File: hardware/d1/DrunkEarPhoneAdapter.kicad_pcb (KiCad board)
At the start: 4 copper layers, 50 x 35 mm, 185 parts, among them J3 SWD, J4 UART, Q1 CSD17577Q3A, Q2 CSD17577Q3A, Q3 DMG1012T-7, SW1 SSSS811101, SW2 DSHP04TS-S, U1 CS43131-CNZR, U10 BLM15PX601SN1D, U11 TPS7A2033PDBVR, U12 TPS7A2018PDBVR, U13 TPS7A2018PDBVR, U14 BLM15PX601SN1D, U15 ESDA25P35-1U1M, U16 ESDA25P35-1U1M, U17 SN74LVC1G32DBVR, U18 TPS22917DBVR, U19 TPS22917DBVR, U2 STM32G0B1VCT6, U20 SN74AVC4T774RSVR, U21 TCA9406DCUR, U3 TS3USB221RSER, U4 TCPP03-M20, U5 TCPP03-M20, U6 ES8327, U7 TPS7A2018PDBVR, U8 TPS7A2033PDBVR, U9 TPS560430XFDBVR, X1 22.5792MHz, X3 24.576MHz

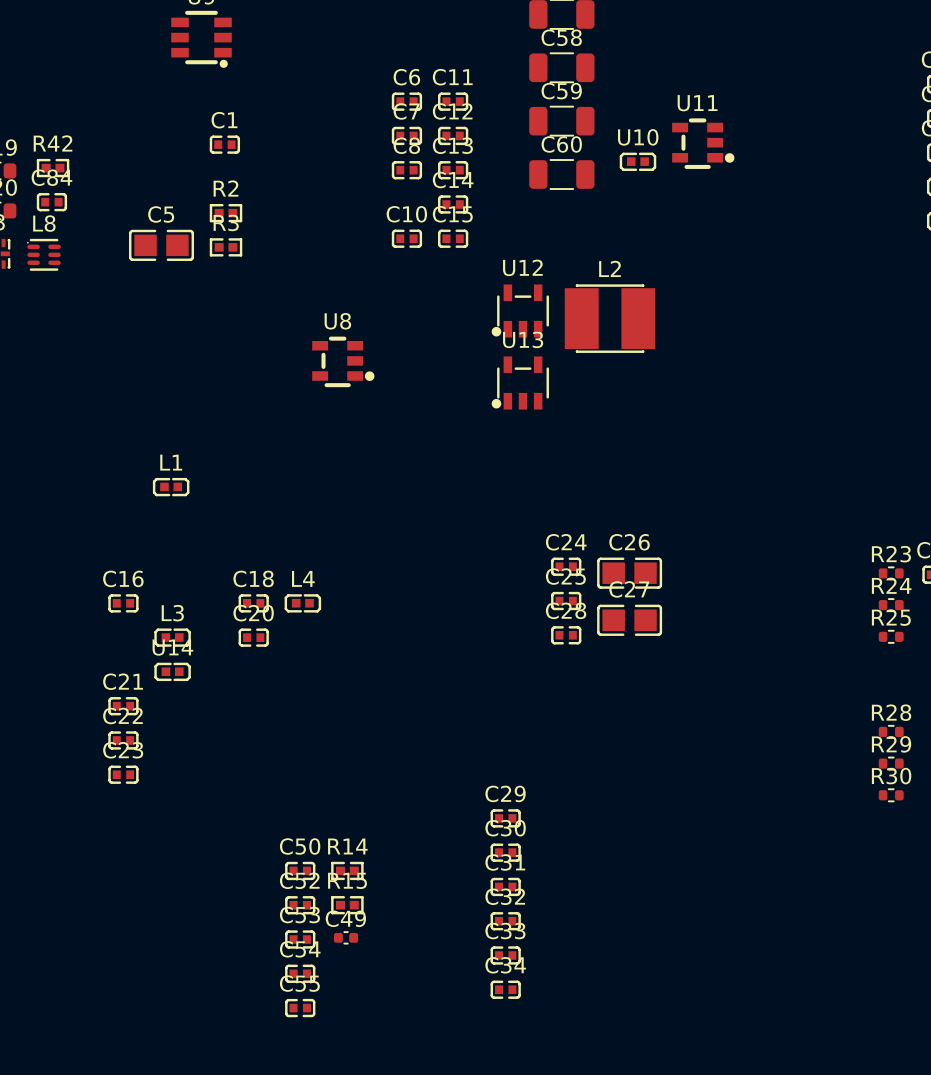
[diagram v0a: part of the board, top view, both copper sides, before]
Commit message: Fix Caps
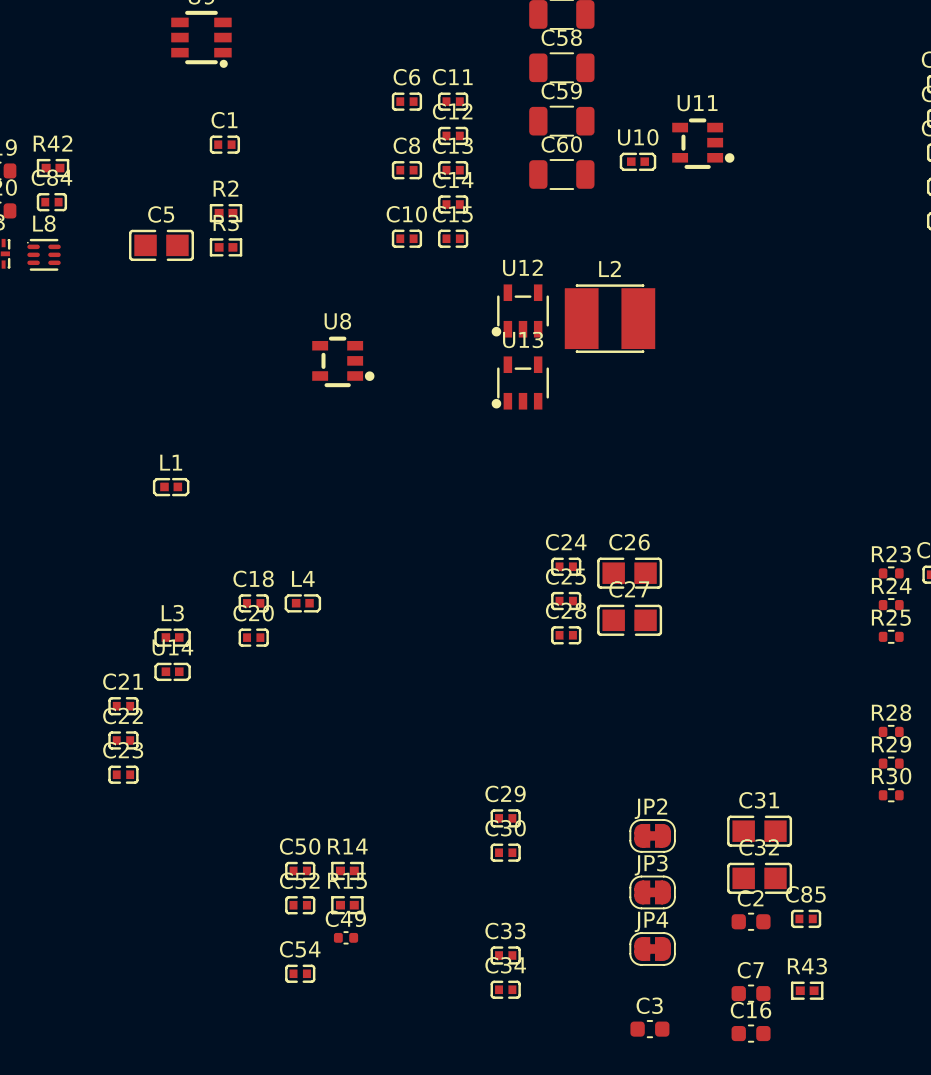
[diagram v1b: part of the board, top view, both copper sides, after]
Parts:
- removed C53, C55: 4.7uF 10V X5R, JLCImport:CL05A475MP5NRNC
- added C2: 4.7uF 10V X5R, Capacitor_SMD:C_0603_1608Metric, F.Cu at (66.9, 124.2)
- added C3: 4.7uF 10V X5R, Capacitor_SMD:C_0603_1608Metric, F.Cu at (60.5, 130.9)
- added C85: 1uF 25V X5R, JLCImport:CL05A105KA5NQNC, F.Cu at (70.3, 124.0)
- added JP2: SolderJumper_2_Bridged, Jumper:SolderJumper-2_P1.3mm_Bridged_RoundedPad1.0x1.5mm, F.Cu at (60.7, 118.8)
- added JP3: SolderJumper_2_Bridged, Jumper:SolderJumper-2_P1.3mm_Bridged_RoundedPad1.0x1.5mm, F.Cu at (60.7, 122.3)
- added JP4: SolderJumper_2_Bridged, Jumper:SolderJumper-2_P1.3mm_Bridged_RoundedPad1.0x1.5mm, F.Cu at (60.7, 125.9)
- added R43: 100kΩ, JLCImport:0402WGF1003TCE, F.Cu at (70.4, 128.5)
- C16, C7: footprint JLCImport:CL05A475MP5NRNC -> Capacitor_SMD:C_0603_1608Metric
- C31, C32: value 2.2uF 16V X5R -> 2.2uF 50V X7R; footprint JLCImport:CL05A225KO5NQNC -> JLCImport:CC0805KKX7R9BB225
- moved C7 58.0 mm to (66.9, 128.7)
- moved C16 47.8 mm to (66.9, 131.2)
- moved C31 16.3 mm to (67.4, 118.5)
- moved C32 16.2 mm to (67.4, 121.4)
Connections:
- C16 pad 1: Net-(U1-VP) -> GND
- C16 pad 2: GND -> +3V3_D
- C32 pad 1: GND -> /dac/VCP_FILT-
- C32 pad 2: /dac/VCP_FILT- -> GND
- C66 pad 1: /ucpd/GDPs -> /ucpd/USB_PHONE_ISENSE
- C7 pad 2: +1V8_D -> +3V3_D
- U4 pad 8: unconnected-(U4-GDCs-Pad8) -> /ucpd/GDCs
- U5 pad 6: unconnected-(U5-GDPs-Pad6) -> /ucpd/GDPs_CHR
- U5 pad 8: unconnected-(U5-GDCs-Pad8) -> /ucpd/GDCs_CHR
